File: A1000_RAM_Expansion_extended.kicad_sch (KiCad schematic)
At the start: 25 parts, among them J1 Front_Connector, J2 Conn_02x05_Odd_Even, U1 XC9572XL-xxVQx64, U2 LD1117S33TR_SOT223

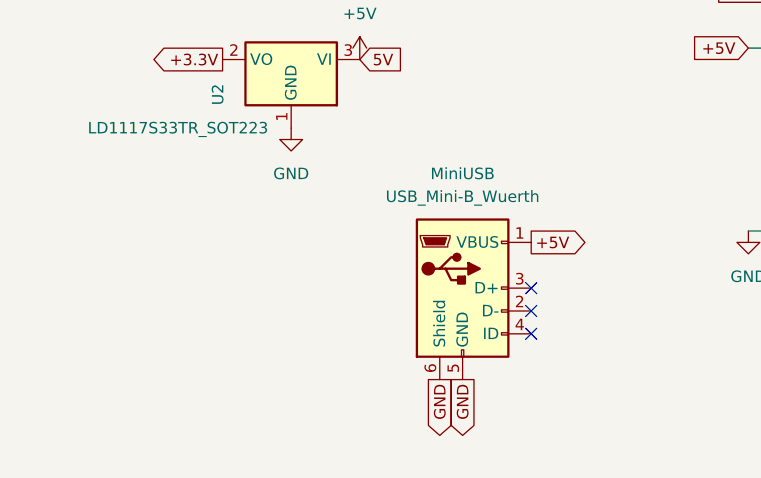
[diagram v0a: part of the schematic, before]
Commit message: Cleanup
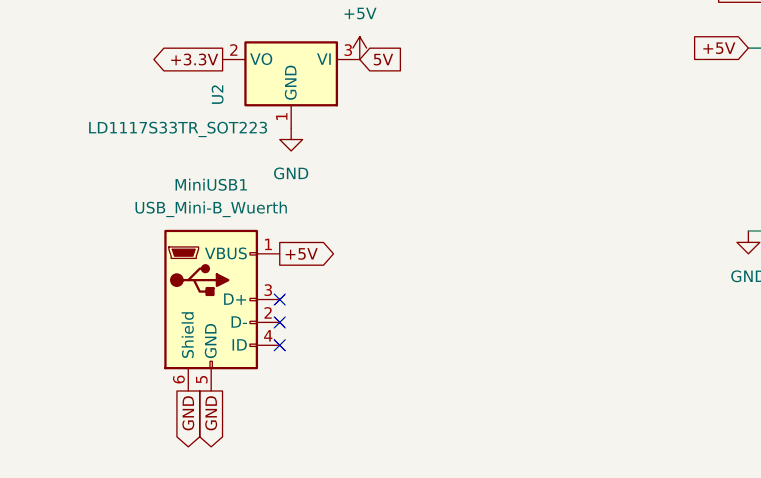
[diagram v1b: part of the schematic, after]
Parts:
- removed MiniUSB: USB_Mini-B_Wuerth, Connector_USB:USB_Mini-B_Wuerth_65100516121_Horizontal, symbol Connector:USB_B_Mini
- added MiniUSB1: USB_Mini-B_Wuerth, Connector_USB:USB_Mini-B_Wuerth_65100516121_Horizontal, symbol Connector:USB_B_Mini
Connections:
- net +5V: now also MiniUSB1.1 (VBUS)
- net GND: now also MiniUSB1.5 (GND), MiniUSB1.6 (Shield)
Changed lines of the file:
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@@
 	)
 	(no_connect
-		(at 72.39 175.26)
-	)
-	(no_connect
 		(at 176.53 96.52)
 	)
@@
 	)
 	(no_connect
+		(at 44.45 171.45)
+	)
+	(no_connect
+		(at 44.45 176.53)
+	)
+	(no_connect
 		(at 207.01 76.2)
 	)
@@
 	)
 	(no_connect
-		(at 72.39 172.72)
+		(at 176.53 99.06)
 	)
 	(no_connect
-		(at 72.39 170.18)
-	)
-	(no_connect
-		(at 176.53 99.06)
+		(at 44.45 173.99)
 	)
 	(bus_entry
@@
 		)
 	)
-	(global_label "+5V"
-		(shape output)
-		(at 72.39 165.1 0)
-		(effects
-			(font
-				(size 1.27 1.27)
-			)
-			(justify left)
-		)
-		(property "Intersheetrefs" "${INTERSHEET_REFS}"
-			(at 72.39 165.1 0)
-			(effects
-				(font
-					(size 1.27 1.27)
-				)
-				(hide yes)
-			)
-		)
-	)
 	(global_label "{slash}CASU1"
 		(shape output)
@@
 		)
 	)
+	(global_label "GND"
+		(shape output)
+		(at 34.29 181.61 270)
+		(effects
+			(font
+				(size 1.27 1.27)
+			)
+			(justify right)
+		)
+		(property "Intersheetrefs" "${INTERSHEET_REFS}"
+			(at 34.29 181.61 0)
+			(effects
+				(font
+					(size 1.27 1.27)
+				)
+				(hide yes)
+			)
+		)
+	)
 	(global_label "DRA1"
 		(shape output)
@@
 		)
 	)
-	(global_label "GND"
-		(shape output)
-		(at 62.23 180.34 270)
-		(effects
-			(font
-				(size 1.27 1.27)
-			)
-			(justify right)
-		)
-		(property "Intersheetrefs" "${INTERSHEET_REFS}"
-			(at 62.23 180.34 0)
-			(effects
-				(font
-					(size 1.27 1.27)
-				)
-				(hide yes)
-			)
-		)
-	)
 	(global_label "DRA3"
 		(shape input)
@@
 		)
 	)
+	(global_label "GND"
+		(shape output)
+		(at 36.83 181.61 270)
+		(effects
+			(font
+				(size 1.27 1.27)
+			)
+			(justify right)
+		)
+		(property "Intersheetrefs" "${INTERSHEET_REFS}"
+			(at 36.83 181.61 0)
+			(effects
+				(font
+					(size 1.27 1.27)
+				)
+				(hide yes)
+			)
+		)
+	)
 	(global_label "sram_a14"
 		(shape input)
@@
 		)
 	)
-	(global_label "GND"
-		(shape output)
-		(at 64.77 180.34 270)
-		(effects
-			(font
-				(size 1.27 1.27)
-			)
-			(justify right)
-		)
-		(property "Intersheetrefs" "${INTERSHEET_REFS}"
-			(at 64.77 180.34 0)
-			(effects
-				(font
-					(size 1.27 1.27)
-				)
-				(hide yes)
-			)
-		)
-	)
 	(global_label "sram_a[0..16]"
 		(shape output)
@@
 		)
 	)
+	(global_label "+5V"
+		(shape output)
+		(at 44.45 166.37 0)
+		(effects
+			(font
+				(size 1.27 1.27)
+			)
+			(justify left)
+		)
+		(property "Intersheetrefs" "${INTERSHEET_REFS}"
+			(at 44.45 166.37 0)
+			(effects
+				(font
+					(size 1.27 1.27)
+				)
+				(hide yes)
+			)
+		)
+	)
 	(global_label "GND"
 		(shape passive)
@@
 	)
 	(symbol
-		(lib_id "Connector:USB_B_Mini")
-		(at 64.77 170.18 0)
+		(lib_id "Device:R_Small")
+		(at 231.14 111.76 90)
 		(unit 1)
 		(exclude_from_sim no)
@@
 		(dnp no)
 		(fields_autoplaced yes)
-		(property "Reference" "MiniUSB"
-			(at 64.77 157.48 0)
+		(property "Reference" "R18"
+			(at 231.14 106.68 90)
 			(effects
 				(font
-					(size 1.27 1.27)
+					(size 1.016 1.016)
 				)
 			)
 		)
-		(property "Value" "USB_Mini-B_Wuerth"
-			(at 64.77 160.02 0)
+		(property "Value" "10K"
+			(at 231.14 109.22 90)
 			(effects
 				(font
@@
 			)
 		)
-		(property "Footprint" "Connector_USB:USB_Mini-B_Wuerth_65100516121_Horizontal"
-			(at 68.58 171.45 0)
+		(property "Footprint" "Resistor_SMD:R_0603_1608Metric_Pad0.98x0.95mm_HandSolder"
+			(at 231.14 111.76 0)
 			(effects
 				(font
@@
 		)
 		(property "Datasheet" "~"
-			(at 68.58 171.45 0)
+			(at 231.14 111.76 0)
 			(effects
 				(font
@@
 			)
 		)
-		(property "Description" "USB Mini Type B connector"
-			(at 64.77 170.18 0)
+		(property "Description" "Resistor, small symbol"
+			(at 231.14 111.76 0)
 			(effects
 				(font
@@
 			)
 		)
-		(pin "5"
-		)
 		(pin "2"
 		)
 		(pin "1"
 		)
-		(pin "4"
-		)
-		(pin "6"
-		)
-		(pin "3"
-		)
 		(instances
-			(project ""
+			(project "A1000_RAM-Expansion"
 				(path "/ac211864-9228-4db4-a24a-88f17cc80a70"
-					(reference "MiniUSB")
+					(reference "R18")
 					(unit 1)
 				)
@@
 	)
 	(symbol
-		(lib_id "Device:R_Small")
-		(at 231.14 111.76 90)
+		(lib_id "Connector:USB_B_Mini")
+		(at 36.83 171.45 0)
 		(unit 1)
 		(exclude_from_sim no)
@@
 		(dnp no)
 		(fields_autoplaced yes)
-		(property "Reference" "R18"
-			(at 231.14 106.68 90)
+		(property "Reference" "MiniUSB1"
+			(at 36.83 158.75 0)
 			(effects
 				(font
-					(size 1.016 1.016)
+					(size 1.27 1.27)
 				)
 			)
 		)
-		(property "Value" "10K"
-			(at 231.14 109.22 90)
+		(property "Value" "USB_Mini-B_Wuerth"
+			(at 36.83 161.29 0)
 			(effects
 				(font
@@
 			)
 		)
-		(property "Footprint" "Resistor_SMD:R_0603_1608Metric_Pad0.98x0.95mm_HandSolder"
-			(at 231.14 111.76 0)
+		(property "Footprint" "Connector_USB:USB_Mini-B_Wuerth_65100516121_Horizontal"
+			(at 40.64 172.72 0)
 			(effects
 				(font
@@
 			)
 		)
-		(property "Datasheet" "~"
-			(at 231.14 111.76 0)
+		(property "Datasheet" ""
+			(at 40.64 172.72 0)
 			(effects
 				(font
@@
 			)
 		)
-		(property "Description" "Resistor, small symbol"
-			(at 231.14 111.76 0)
+		(property "Description" ""
+			(at 36.83 171.45 0)
 			(effects
 				(font
@@
 			)
 		)
-		(pin "2"
+		(pin "6"
+		)
+		(pin "4"
+		)
+		(pin "3"
 		)
 		(pin "1"
 		)
+		(pin "2"
+		)
+		(pin "5"
+		)
 		(instances
-			(project "A1000_RAM-Expansion"
+			(project ""
 				(path "/ac211864-9228-4db4-a24a-88f17cc80a70"
-					(reference "R18")
+					(reference "MiniUSB1")
 					(unit 1)
 				)
